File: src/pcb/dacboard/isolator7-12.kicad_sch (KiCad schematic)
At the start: 18 parts, among them U89 ISO7761FQDBQRQ1, U90 ISO7761FQDBQRQ1, U91 ISO7761FQDBQRQ1, U92 ISO7761FQDBQRQ1, U93 ISO7761FQDBQRQ1, U94 ISO7761FQDBQRQ1

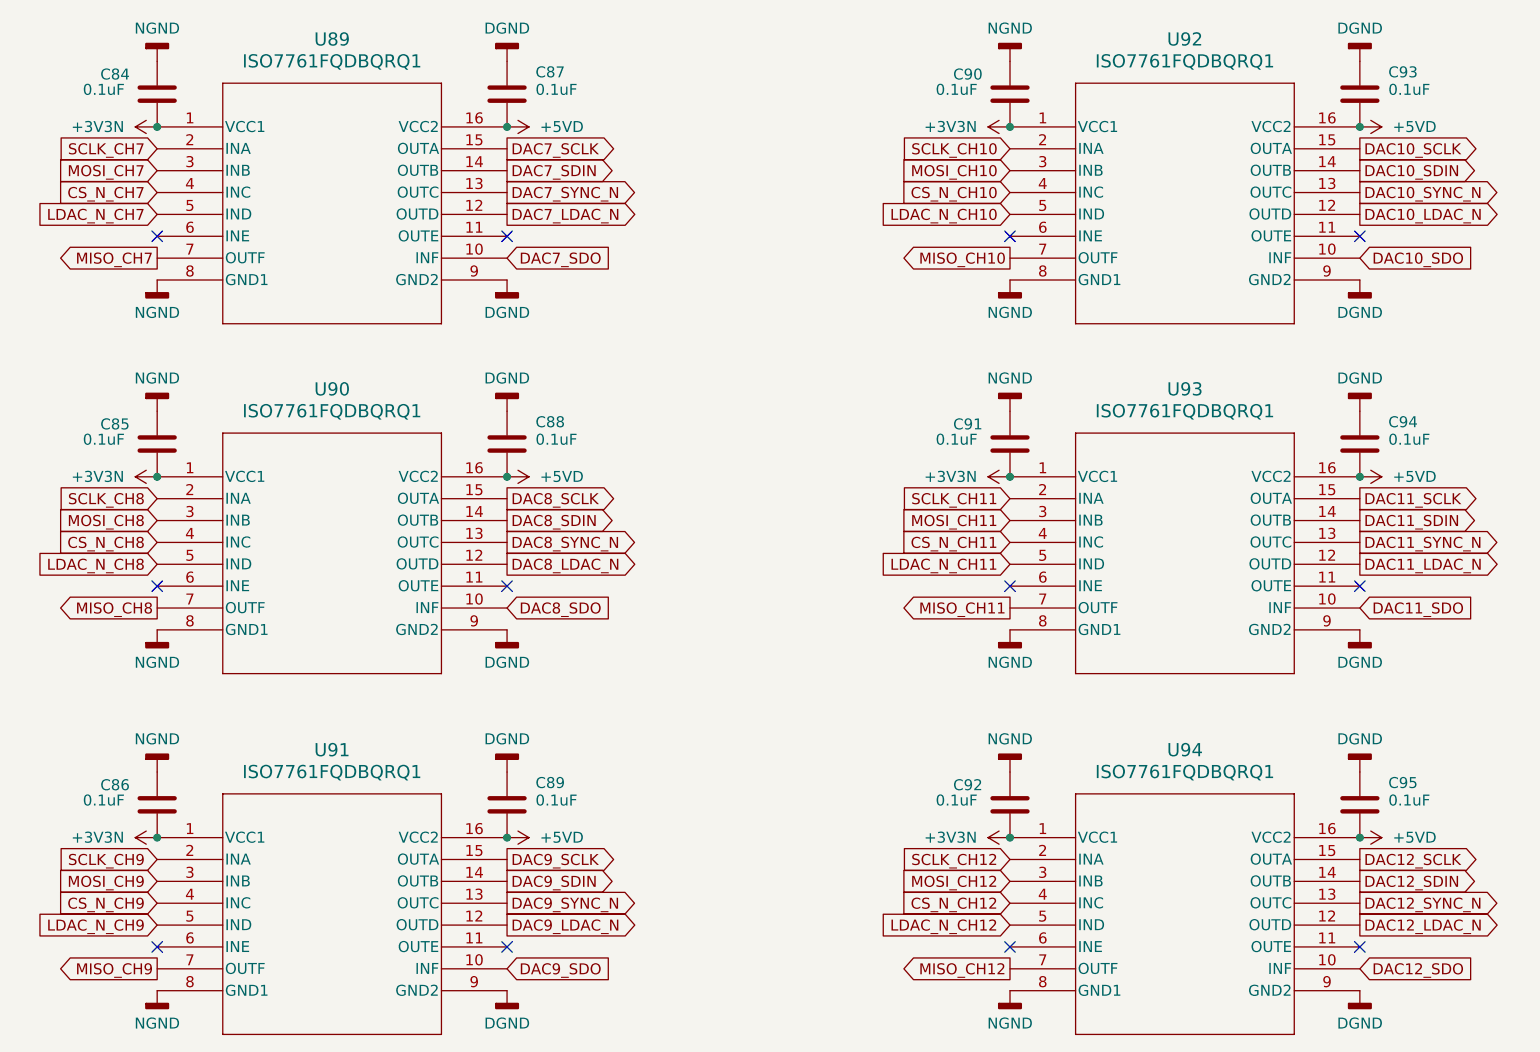
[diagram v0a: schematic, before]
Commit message: dacboard routing
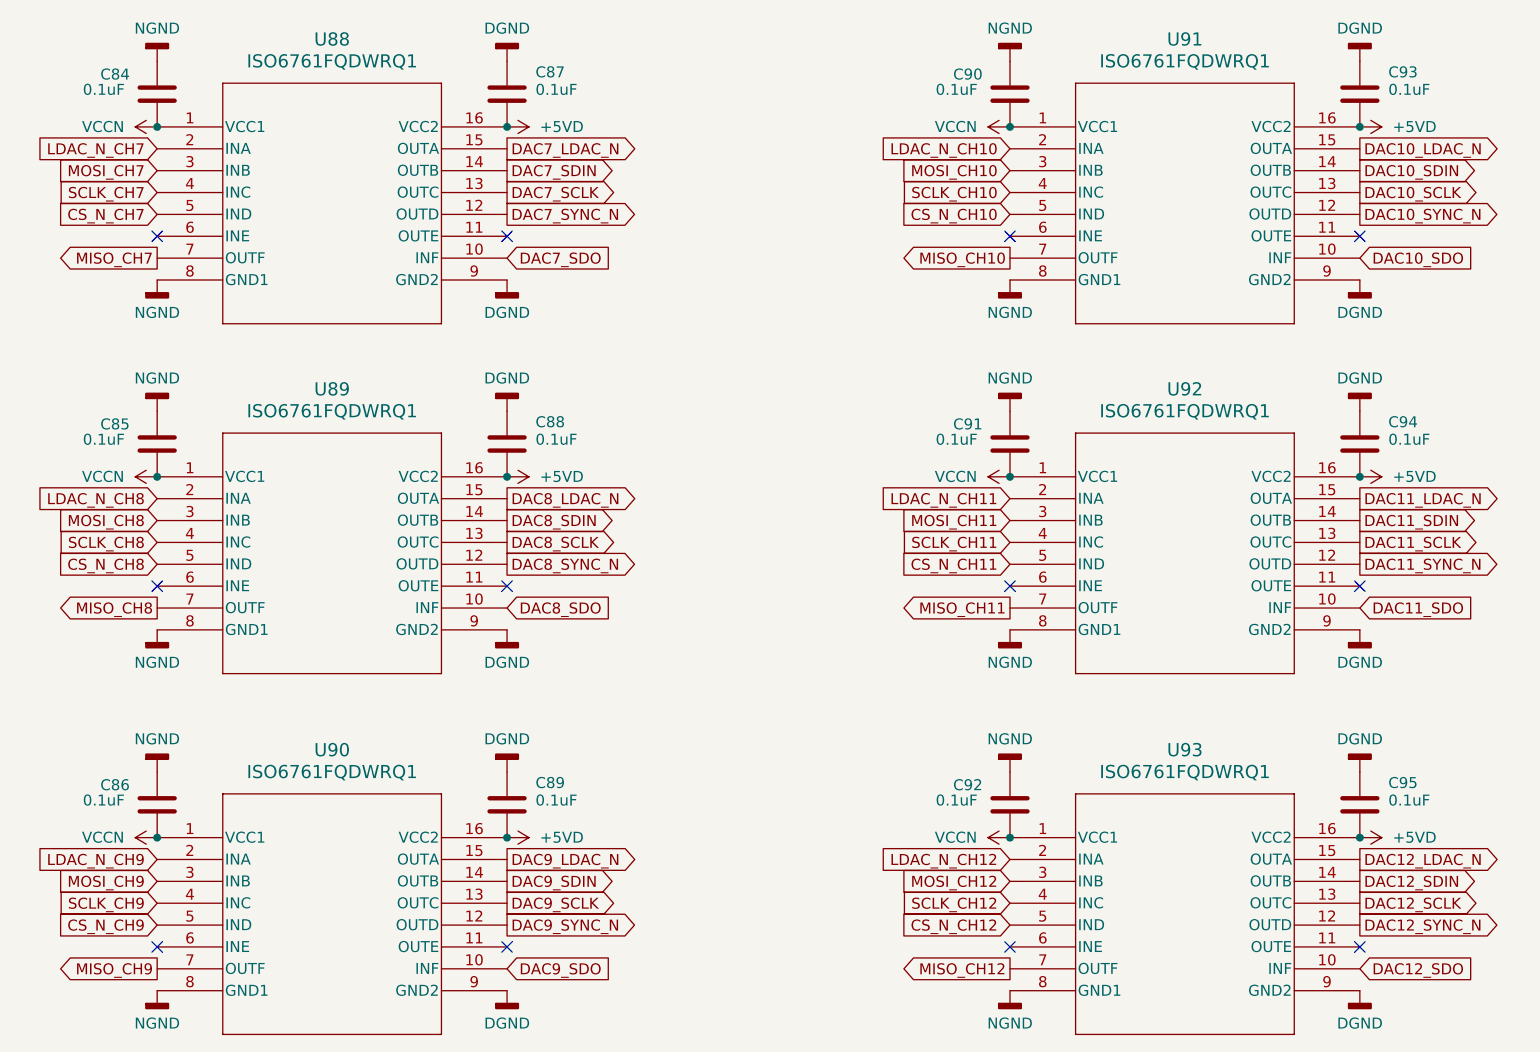
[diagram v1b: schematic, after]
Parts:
- removed U89, U90, U91, U92, U93, U94: ISO7761FQDBQRQ1, DBQ16_TEX, symbol 2025-11-18_20-36-36:ISO7761FQDBQRQ1
- added U88, U89, U90, U91, U92, U93: ISO6761FQDWRQ1, ISO6761:SOIC16_DW_TEX, symbol 2025-11-20_00-47-15:ISO6761FQDWRQ1
- C84, C85, C86, C87, C88, C89, C90, C91, C92, C93, C94, C95: footprint (none) -> Capacitor_SMD:C_0402_1005Metric_Pad0.74x0.62mm_HandSolder
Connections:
- net +5VD: now also U88.16 (VCC2), U89.16 (VCC2), U90.16 (VCC2), U91.16 (VCC2), U92.16 (VCC2), U93.16 (VCC2)
- net CS_N_CH10: now also U91.5 (IND)
- net CS_N_CH11: now also U92.5 (IND)
- net CS_N_CH12: now also U93.5 (IND)
- net CS_N_CH7: now also U88.5 (IND)
- net CS_N_CH8: now also U89.5 (IND)
- net CS_N_CH9: now also U90.5 (IND)
- net DAC10_LDAC_N: now also U91.15 (OUTA)
- net DAC10_SCLK: now also U91.13 (OUTC)
- net DAC10_SDIN: now also U91.14 (OUTB)
- net DAC10_SDO: now also U91.10 (INF)
- net DAC10_SYNC_N: now also U91.12 (OUTD)
- net DAC11_LDAC_N: now also U92.15 (OUTA)
- net DAC11_SCLK: now also U92.13 (OUTC)
- net DAC11_SDIN: now also U92.14 (OUTB)
- net DAC11_SDO: now also U92.10 (INF)
- net DAC11_SYNC_N: now also U92.12 (OUTD)
- net DAC12_LDAC_N: now also U93.15 (OUTA)
- net DAC12_SCLK: now also U93.13 (OUTC)
- net DAC12_SDIN: now also U93.14 (OUTB)
- net DAC12_SDO: now also U93.10 (INF)
- net DAC12_SYNC_N: now also U93.12 (OUTD)
- net DAC7_LDAC_N: now also U88.15 (OUTA)
- net DAC7_SCLK: now also U88.13 (OUTC)
- net DAC7_SDIN: now also U88.14 (OUTB)
- net DAC7_SDO: now also U88.10 (INF)
- net DAC7_SYNC_N: now also U88.12 (OUTD)
- net DAC8_LDAC_N: now also U89.15 (OUTA)
- net DAC8_SCLK: now also U89.13 (OUTC)
- net DAC8_SDIN: now also U89.14 (OUTB)
- net DAC8_SDO: now also U89.10 (INF)
- net DAC8_SYNC_N: now also U89.12 (OUTD)
- net DAC9_LDAC_N: now also U90.15 (OUTA)
- net DAC9_SCLK: now also U90.13 (OUTC)
- net DAC9_SDIN: now also U90.14 (OUTB)
- net DAC9_SDO: now also U90.10 (INF)
- net DAC9_SYNC_N: now also U90.12 (OUTD)
- net DGND: now also U88.9 (GND2), U89.9 (GND2), U90.9 (GND2), U91.9 (GND2), U92.9 (GND2), U93.9 (GND2)
- net LDAC_N_CH10: now also U91.2 (INA)
- net LDAC_N_CH11: now also U92.2 (INA)
- net LDAC_N_CH12: now also U93.2 (INA)
- net LDAC_N_CH7: now also U88.2 (INA)
- net LDAC_N_CH8: now also U89.2 (INA)
- net LDAC_N_CH9: now also U90.2 (INA)
- net MISO_CH10: now also U91.7 (OUTF)
- net MISO_CH11: now also U92.7 (OUTF)
- net MISO_CH12: now also U93.7 (OUTF)
- net MISO_CH7: now also U88.7 (OUTF)
- net MISO_CH8: now also U89.7 (OUTF)
- net MISO_CH9: now also U90.7 (OUTF)
- net MOSI_CH10: now also U91.3 (INB)
- net MOSI_CH11: now also U92.3 (INB)
- net MOSI_CH12: now also U93.3 (INB)
- net MOSI_CH7: now also U88.3 (INB)
- net MOSI_CH8: now also U89.3 (INB)
- net MOSI_CH9: now also U90.3 (INB)
- net NGND: now also U88.8 (GND1), U89.8 (GND1), U90.8 (GND1), U91.8 (GND1), U92.8 (GND1), U93.8 (GND1)
- net SCLK_CH10: now also U91.4 (INC)
- net SCLK_CH11: now also U92.4 (INC)
- net SCLK_CH12: now also U93.4 (INC)
- net SCLK_CH7: now also U88.4 (INC)
- net SCLK_CH8: now also U89.4 (INC)
- net SCLK_CH9: now also U90.4 (INC)
- net +3V3N renamed VCCN
- net VCCN: now also U88.1 (VCC1), U89.1 (VCC1), U90.1 (VCC1), U91.1 (VCC1), U92.1 (VCC1), U93.1 (VCC1)

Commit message: adding more capacitors to analog side
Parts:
- U88, U89, U90, U91, U92, U93: footprint ISO6761:SOIC16_DW_TEX -> Package_SO:SOIC-16W_7.5x10.3mm_P1.27mm
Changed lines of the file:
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@@
 			)
 		)
-		(property "Footprint" "ISO6761:SOIC16_DW_TEX"
+		(property "Footprint" "Package_SO:SOIC-16W_7.5x10.3mm_P1.27mm"
 			(at 78.74 41.91 0)
 			(effects
@@
 			)
 		)
-		(property "Footprint" "ISO6761:SOIC16_DW_TEX"
+		(property "Footprint" "Package_SO:SOIC-16W_7.5x10.3mm_P1.27mm"
 			(at 177.8 124.46 0)
 			(effects
@@
 			)
 		)
-		(property "Footprint" "ISO6761:SOIC16_DW_TEX"
+		(property "Footprint" "Package_SO:SOIC-16W_7.5x10.3mm_P1.27mm"
 			(at 177.8 41.91 0)
 			(effects
@@
 			)
 		)
-		(property "Footprint" "ISO6761:SOIC16_DW_TEX"
+		(property "Footprint" "Package_SO:SOIC-16W_7.5x10.3mm_P1.27mm"
 			(at 78.74 82.55 0)
 			(effects
@@
 			)
 		)
-		(property "Footprint" "ISO6761:SOIC16_DW_TEX"
+		(property "Footprint" "Package_SO:SOIC-16W_7.5x10.3mm_P1.27mm"
 			(at 78.74 124.46 0)
 			(effects
@@
 			)
 		)
-		(property "Footprint" "ISO6761:SOIC16_DW_TEX"
+		(property "Footprint" "Package_SO:SOIC-16W_7.5x10.3mm_P1.27mm"
 			(at 177.8 82.55 0)
 			(effects
